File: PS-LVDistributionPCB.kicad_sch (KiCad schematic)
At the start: 4 parts

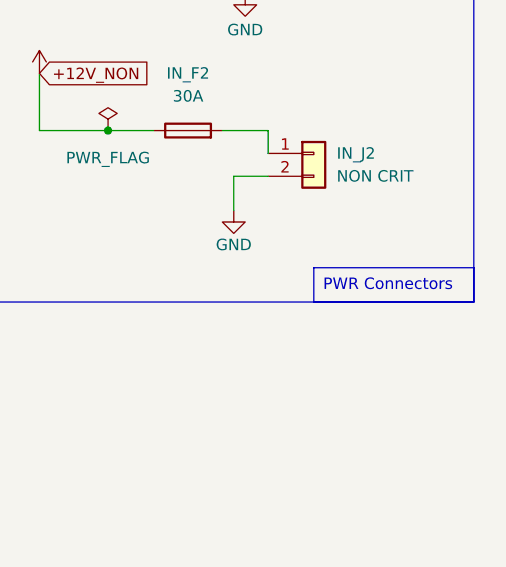
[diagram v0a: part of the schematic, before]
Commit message: solder bridges
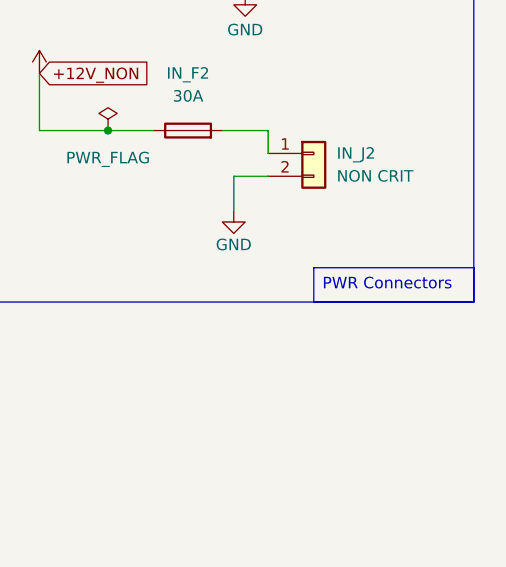
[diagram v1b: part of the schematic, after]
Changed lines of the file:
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@@
 (kicad_sch
-	(version 20231120)
+	(version 20250114)
 	(generator "eeschema")
-	(generator_version "8.0")
+	(generator_version "9.0")
 	(paper "A4")
+	(rectangle
+		(start 153.67 120.65)
+		(end 175.26 125.73)
+		(stroke
+			(width 0)
+			(type default)
+		)
+		(fill
+			(type none)
+		)
+	)
+	(rectangle
+		(start 186.69 31.75)
+		(end 243.84 90.17)
+		(stroke
+			(width 0)
+			(type default)
+		)
+		(fill
+			(type none)
+		)
+	)
+	(rectangle
+		(start 49.53 31.75)
+		(end 88.9 139.7)
+		(stroke
+			(width 0)
+			(type default)
+		)
+		(fill
+			(type none)
+		)
+	)
+	(rectangle
+		(start 72.39 134.112)
+		(end 88.9 139.7)
+		(stroke
+			(width 0)
+			(type default)
+		)
+		(fill
+			(type none)
+		)
+	)
+	(rectangle
+		(start 101.6 31.75)
+		(end 175.26 125.73)
+		(stroke
+			(width 0)
+			(type default)
+		)
+		(fill
+			(type none)
+		)
+	)
+	(text "Non Critical Fuses"
+		(exclude_from_sim no)
+		(at 164.338 123.444 0)
+		(effects
+			(font
+				(size 1.27 1.27)
+			)
+		)
+	)
+	(text "Critical Fuses"
+		(exclude_from_sim no)
+		(at 80.772 137.16 0)
+		(effects
+			(font
+				(size 1.27 1.27)
+			)
+		)
+	)
+	(text_box "PWR Connectors"
+		(exclude_from_sim no)
+		(at 226.06 86.36 0)
+		(size 17.78 3.81)
+		(margins 0.9525 0.9525 0.9525 0.9525)
+		(stroke
+			(width 0)
+			(type default)
+		)
+		(fill
+			(type none)
+		)
+		(effects
+			(font
+				(size 1.27 1.27)
+			)
+			(justify left top)
+		)
+	)
 	(junction
 		(at 204.47 46.99)
@@
 			(width 0)
 			(type default)
-		)
-	)
-	(rectangle
-		(start 153.67 120.65)
-		(end 175.26 125.73)
-		(stroke
-			(width 0)
-			(type default)
-		)
-		(fill
-			(type none)
-		)
-	)
-	(rectangle
-		(start 186.69 31.75)
-		(end 243.84 90.17)
-		(stroke
-			(width 0)
-			(type default)
-		)
-		(fill
-			(type none)
-		)
-	)
-	(rectangle
-		(start 49.53 31.75)
-		(end 88.9 139.7)
-		(stroke
-			(width 0)
-			(type default)
-		)
-		(fill
-			(type none)
-		)
-	)
-	(rectangle
-		(start 72.39 134.112)
-		(end 88.9 139.7)
-		(stroke
-			(width 0)
-			(type default)
-		)
-		(fill
-			(type none)
-		)
-	)
-	(rectangle
-		(start 101.6 31.75)
-		(end 175.26 125.73)
-		(stroke
-			(width 0)
-			(type default)
-		)
-		(fill
-			(type none)
-		)
-	)
-	(text_box "PWR Connectors"
-		(exclude_from_sim no)
-		(at 226.06 86.36 0)
-		(size 17.78 3.81)
-		(stroke
-			(width 0)
-			(type default)
-		)
-		(fill
-			(type none)
-		)
-		(effects
-			(font
-				(size 1.27 1.27)
-			)
-			(justify left top)
-		)
-	)
-	(text "Non Critical Fuses"
-		(exclude_from_sim no)
-		(at 164.338 123.444 0)
-		(effects
-			(font
-				(size 1.27 1.27)
-			)
-		)
-	)
-	(text "Critical Fuses"
-		(exclude_from_sim no)
-		(at 80.772 137.16 0)
-		(effects
-			(font
-				(size 1.27 1.27)
-			)
 		)
 	)
@@
 		(at 54.61 80.01)
 		(size 29.21 7.62)
+		(exclude_from_sim no)
+		(in_bom yes)
+		(on_board yes)
+		(dnp no)
 		(fields_autoplaced yes)
 		(stroke
@@
 		(at 140.97 66.04)
 		(size 29.21 7.62)
+		(exclude_from_sim no)
+		(in_bom yes)
+		(on_board yes)
+		(dnp no)
 		(stroke
 			(width 0.1524)
@@
 		(at 106.68 80.01)
 		(size 29.21 7.62)
+		(exclude_from_sim no)
+		(in_bom yes)
+		(on_board yes)
+		(dnp no)
 		(stroke
 			(width 0.1524)
@@
 		(at 54.61 93.98)
 		(size 29.21 7.62)
+		(exclude_from_sim no)
+		(in_bom yes)
+		(on_board yes)
+		(dnp no)
 		(fields_autoplaced yes)
 		(stroke
@@
 		(at 54.61 107.95)
 		(size 29.21 7.62)
+		(exclude_from_sim no)
+		(in_bom yes)
+		(on_board yes)
+		(dnp no)
 		(fields_autoplaced yes)
 		(stroke
@@
 		(at 54.61 66.04)
 		(size 29.21 7.62)
+		(exclude_from_sim no)
+		(in_bom yes)
+		(on_board yes)
+		(dnp no)
 		(fields_autoplaced yes)
 		(stroke
@@
 		(at 140.97 38.1)
 		(size 29.21 7.62)
+		(exclude_from_sim no)
+		(in_bom yes)
+		(on_board yes)
+		(dnp no)
 		(stroke
 			(width 0.1524)
@@
 		(at 140.97 80.01)
 		(size 29.21 7.62)
+		(exclude_from_sim no)
+		(in_bom yes)
+		(on_board yes)
+		(dnp no)
 		(stroke
 			(width 0.1524)
@@
 		(at 106.68 52.07)
 		(size 29.21 7.62)
+		(exclude_from_sim no)
+		(in_bom yes)
+		(on_board yes)
+		(dnp no)
 		(stroke
 			(width 0.1524)
@@
 		(at 140.97 107.95)
 		(size 29.21 7.62)
+		(exclude_from_sim no)
+		(in_bom yes)
+		(on_board yes)
+		(dnp no)
 		(stroke
 			(width 0.1524)
@@
 		(at 140.97 52.07)
 		(size 29.21 7.62)
+		(exclude_from_sim no)
+		(in_bom yes)
+		(on_board yes)
+		(dnp no)
 		(stroke
 			(width 0.1524)
@@
 		(at 54.61 121.92)
 		(size 29.21 7.62)
+		(exclude_from_sim no)
+		(in_bom yes)
+		(on_board yes)
+		(dnp no)
 		(fields_autoplaced yes)
 		(stroke
@@
 		(at 106.68 66.04)
 		(size 29.21 7.62)
+		(exclude_from_sim no)
+		(in_bom yes)
+		(on_board yes)
+		(dnp no)
 		(stroke
 			(width 0.1524)
@@
 		(at 54.61 38.1)
 		(size 29.21 7.62)
+		(exclude_from_sim no)
+		(in_bom yes)
+		(on_board yes)
+		(dnp no)
 		(fields_autoplaced yes)
 		(stroke
@@
 		(at 106.68 107.95)
 		(size 29.21 7.62)
+		(exclude_from_sim no)
+		(in_bom yes)
+		(on_board yes)
+		(dnp no)
 		(stroke
 			(width 0.1524)
@@
 		(at 54.61 52.07)
 		(size 29.21 7.62)
+		(exclude_from_sim no)
+		(in_bom yes)
+		(on_board yes)
+		(dnp no)
 		(fields_autoplaced yes)
 		(stroke
@@
 		(at 106.68 93.98)
 		(size 29.21 7.62)
+		(exclude_from_sim no)
+		(in_bom yes)
+		(on_board yes)
+		(dnp no)
 		(stroke
 			(width 0.1524)
@@
 		(at 106.68 38.1)
 		(size 29.21 7.62)
+		(exclude_from_sim no)
+		(in_bom yes)
+		(on_board yes)
+		(dnp no)
 		(stroke
 			(width 0.1524)
@@
 		(at 140.97 93.98)
 		(size 29.21 7.62)
+		(exclude_from_sim no)
+		(in_bom yes)
+		(on_board yes)
+		(dnp no)
 		(stroke
 			(width 0.1524)
@@
 		)
 	)
+	(embedded_fonts no)
 )
